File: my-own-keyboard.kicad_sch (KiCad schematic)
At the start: 140 parts, among them J2 5077CR-16SMC2-BK-TR, SW1 Reset SW, SW10 8, SW11 9, SW12 0, SW13 -, SW14 =, SW15 Backspace, SW16 Tab, SW17 Q, SW18 W, SW19 E, SW2 `, SW20 R, SW21 T, SW22 Y, SW23 U, SW24 I, SW25 O, SW26 P, SW27 [, SW28 ], SW29 \, SW3 1, SW30 Capslock, SW31 A, SW32 S, SW33 D, SW34 F, SW35 G, SW36 H, SW37 J, SW38 K, SW39 L, SW4 2, SW40 ;, SW41 ', SW42 Enter, SW43 L-shift, SW44 Z, SW45 X, SW46 C, SW47 V, SW48 B, SW49 N, SW5 3, SW50 M, SW51 ,, SW52 ., SW53 /, SW54 R-shift, SW55 L-Ctrl, SW56 win, SW57 L-Alt, SW58 Space, SW59 Fn, SW6 4, SW60 R-Alt, SW61 Menu, SW62 R-Ctrl, SW63 RotaryEncoder_Switch, SW7 5, SW8 6, SW9 7, U1 ATmega32U4-A, Y1 16MHz

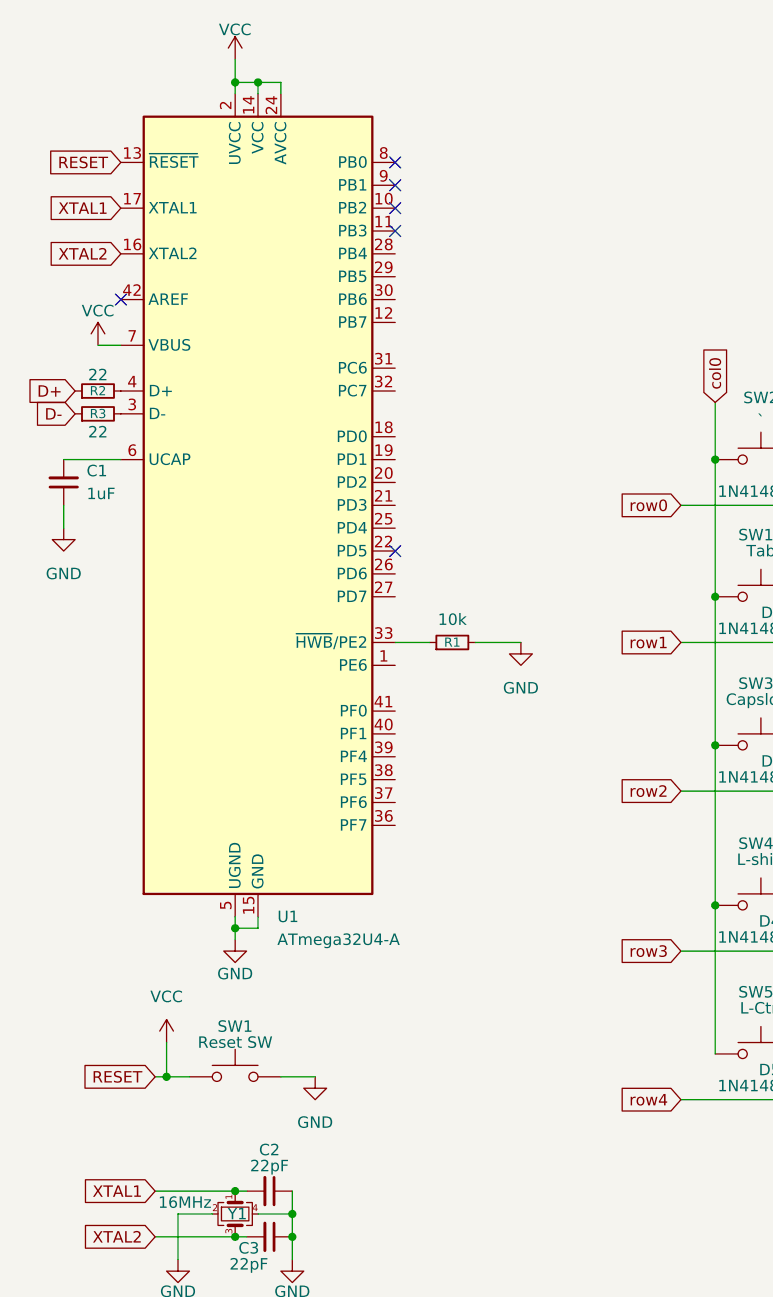
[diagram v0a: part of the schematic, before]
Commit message: wired
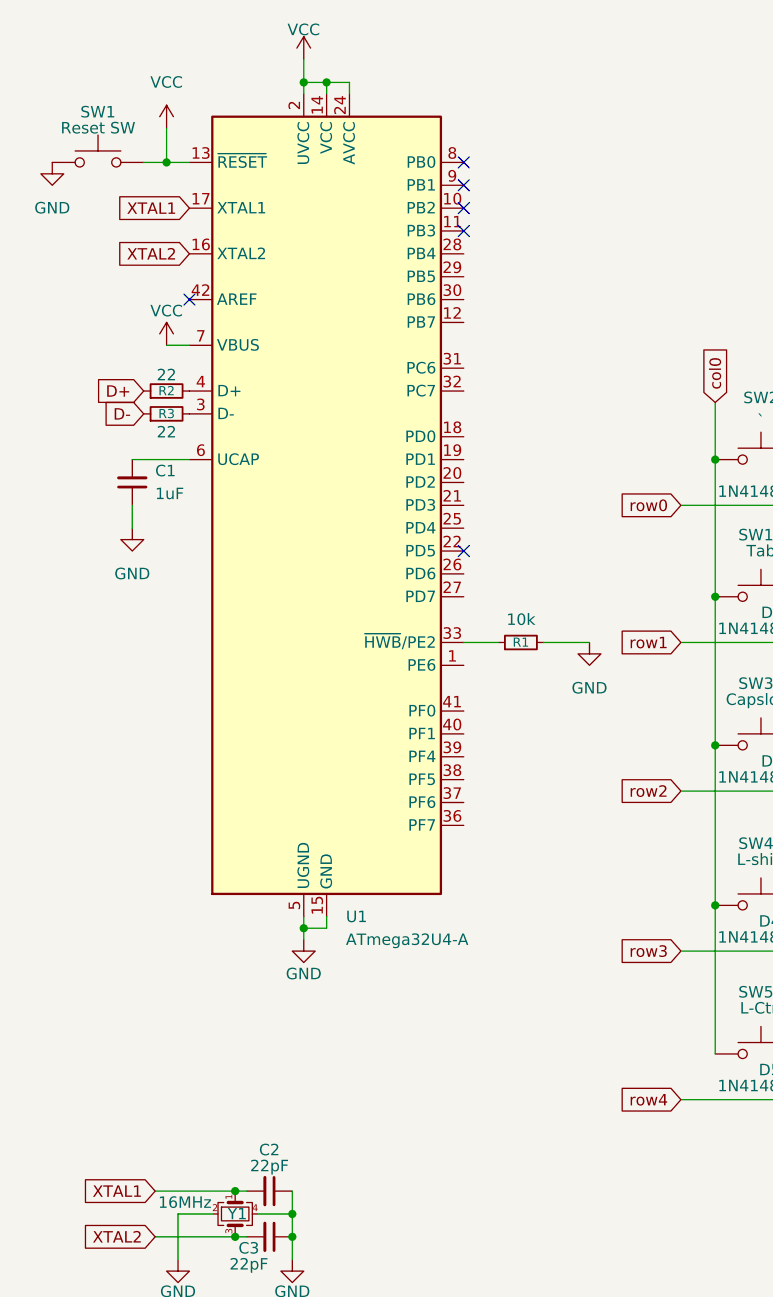
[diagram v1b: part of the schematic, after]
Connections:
- net GND: now also SW1.1; no longer SW1.2
- net VCC: now also SW1.2; no longer SW1.1
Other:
- moved on the sheet: C1, R1, R2, R3, SW1, U1

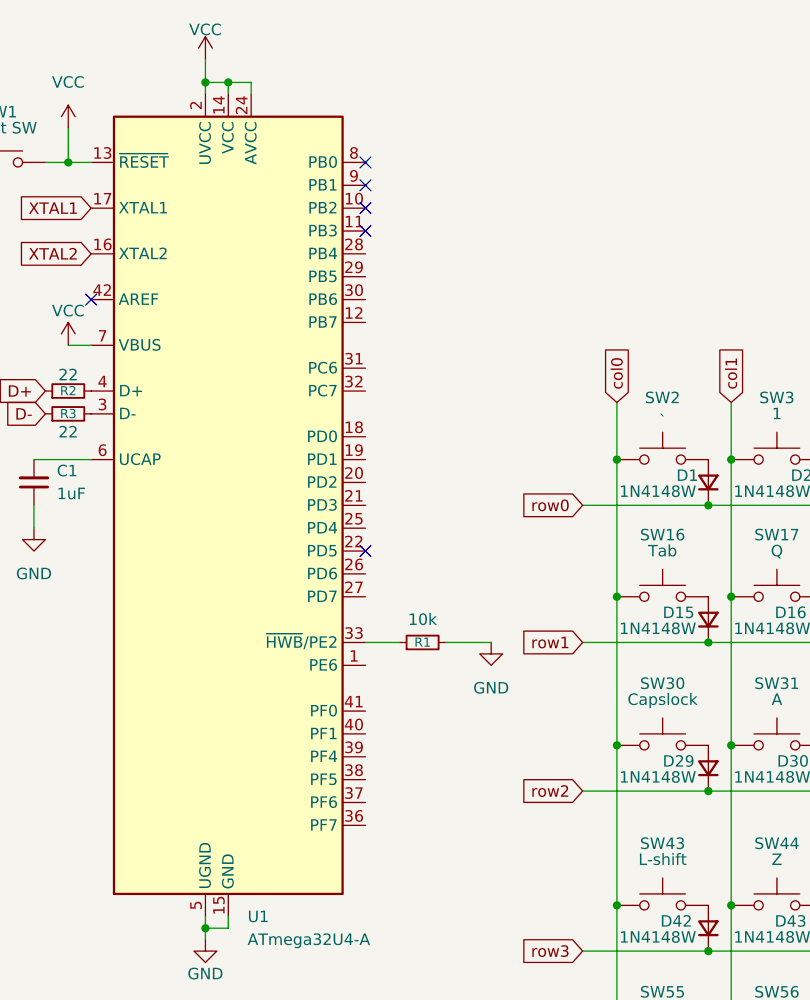
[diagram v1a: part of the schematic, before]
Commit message: completed wiring
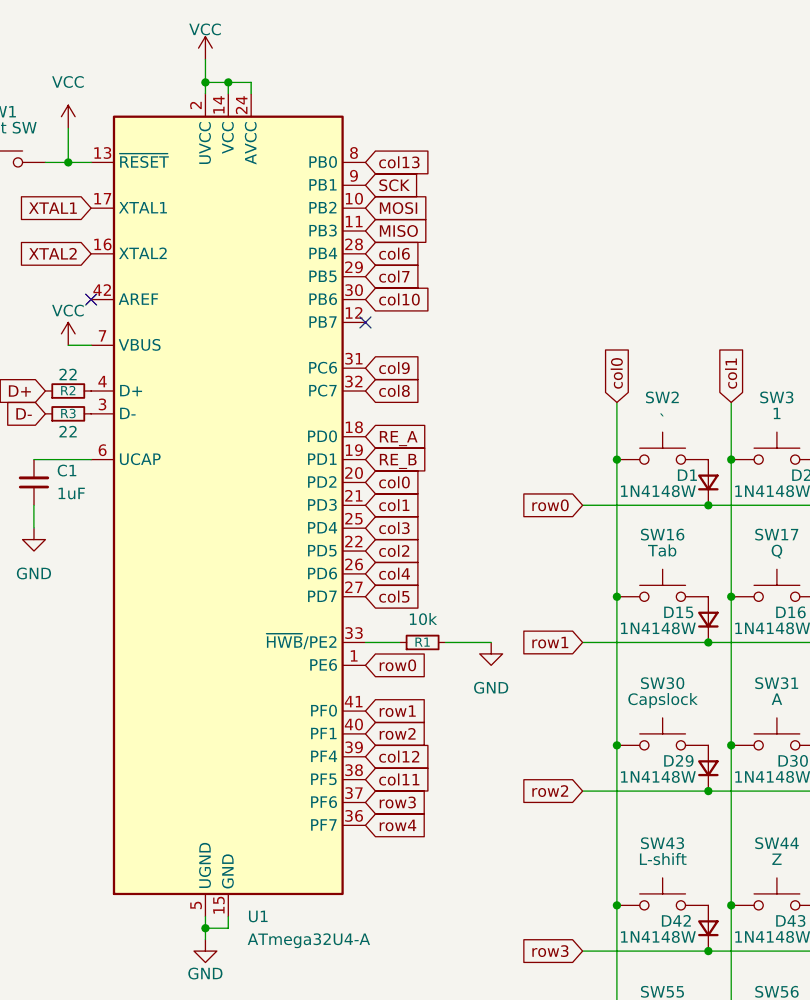
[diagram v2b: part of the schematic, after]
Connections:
- net RE_A: now also U1.18 (PD0)
- net RE_B: now also U1.19 (PD1)
- net col0: now also U1.20 (PD2)
- net col1: now also U1.21 (PD3)
- net col10: now also U1.30 (PB6)
- net col11: now also U1.38 (PF5)
- net col12: now also U1.39 (PF4)
- net col13: now also U1.8 (PB0)
- net col2: now also U1.22 (PD5)
- net col3: now also U1.25 (PD4)
- net col4: now also U1.26 (PD6)
- net col5: now also U1.27 (PD7)
- net col6: now also U1.28 (PB4)
- net col7: now also U1.29 (PB5)
- net col8: now also U1.32 (PC7)
- net col9: now also U1.31 (PC6)
- net row0: now also U1.1 (PE6)
- net row1: now also U1.41 (PF0)
- net row2: now also U1.40 (PF1)
- net row3: now also U1.37 (PF6)
- net row4: now also U1.36 (PF7)
- net MOSI: now reaches U1.10 (PB2)
- net MISO: now reaches U1.11 (PB3)
- net SCK: now reaches U1.9 (PB1)
- no-connect marks 8 -> 4
